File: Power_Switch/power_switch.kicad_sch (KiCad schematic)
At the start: 24 parts, among them J1 Conn_01x03_Pin, J2 GCT_FFC2B28-12-G, J6 Conn_01x02_Pin, Q9 2N7002, SW1 SW_SPDT, U6 BQ24075RGT

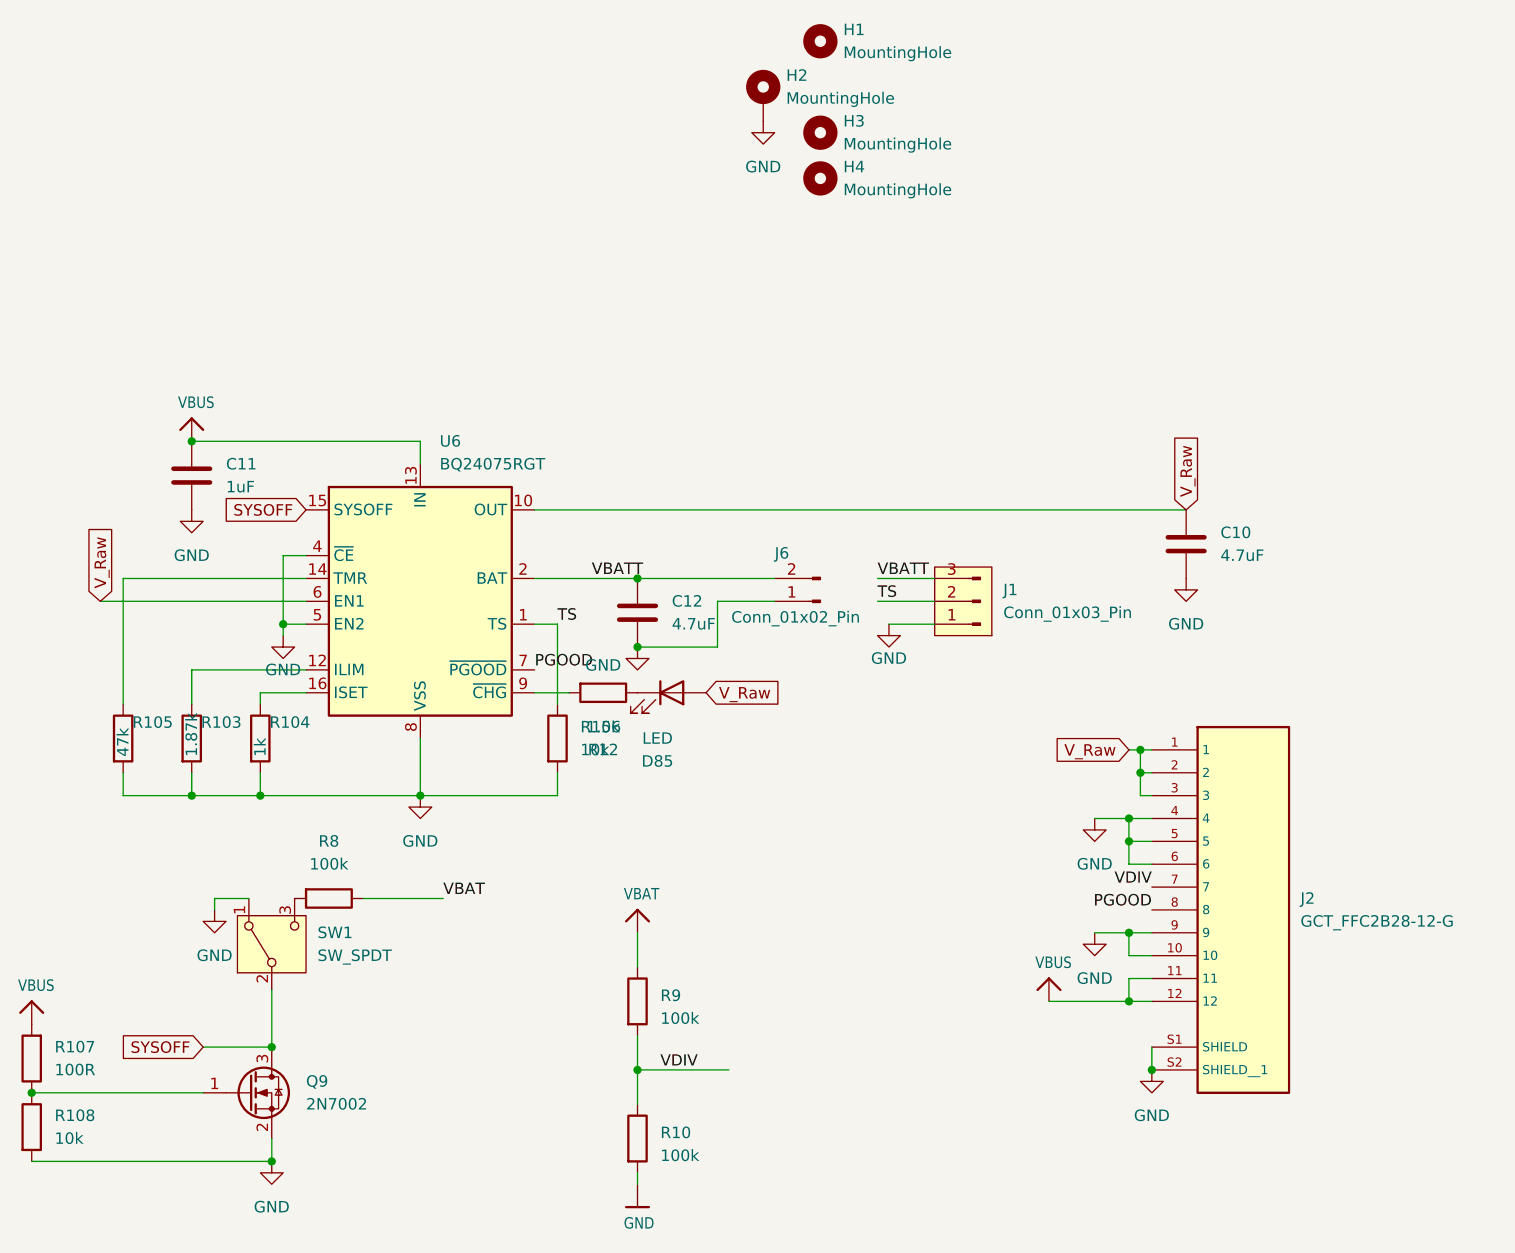
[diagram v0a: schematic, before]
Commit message: Work on Power Switch
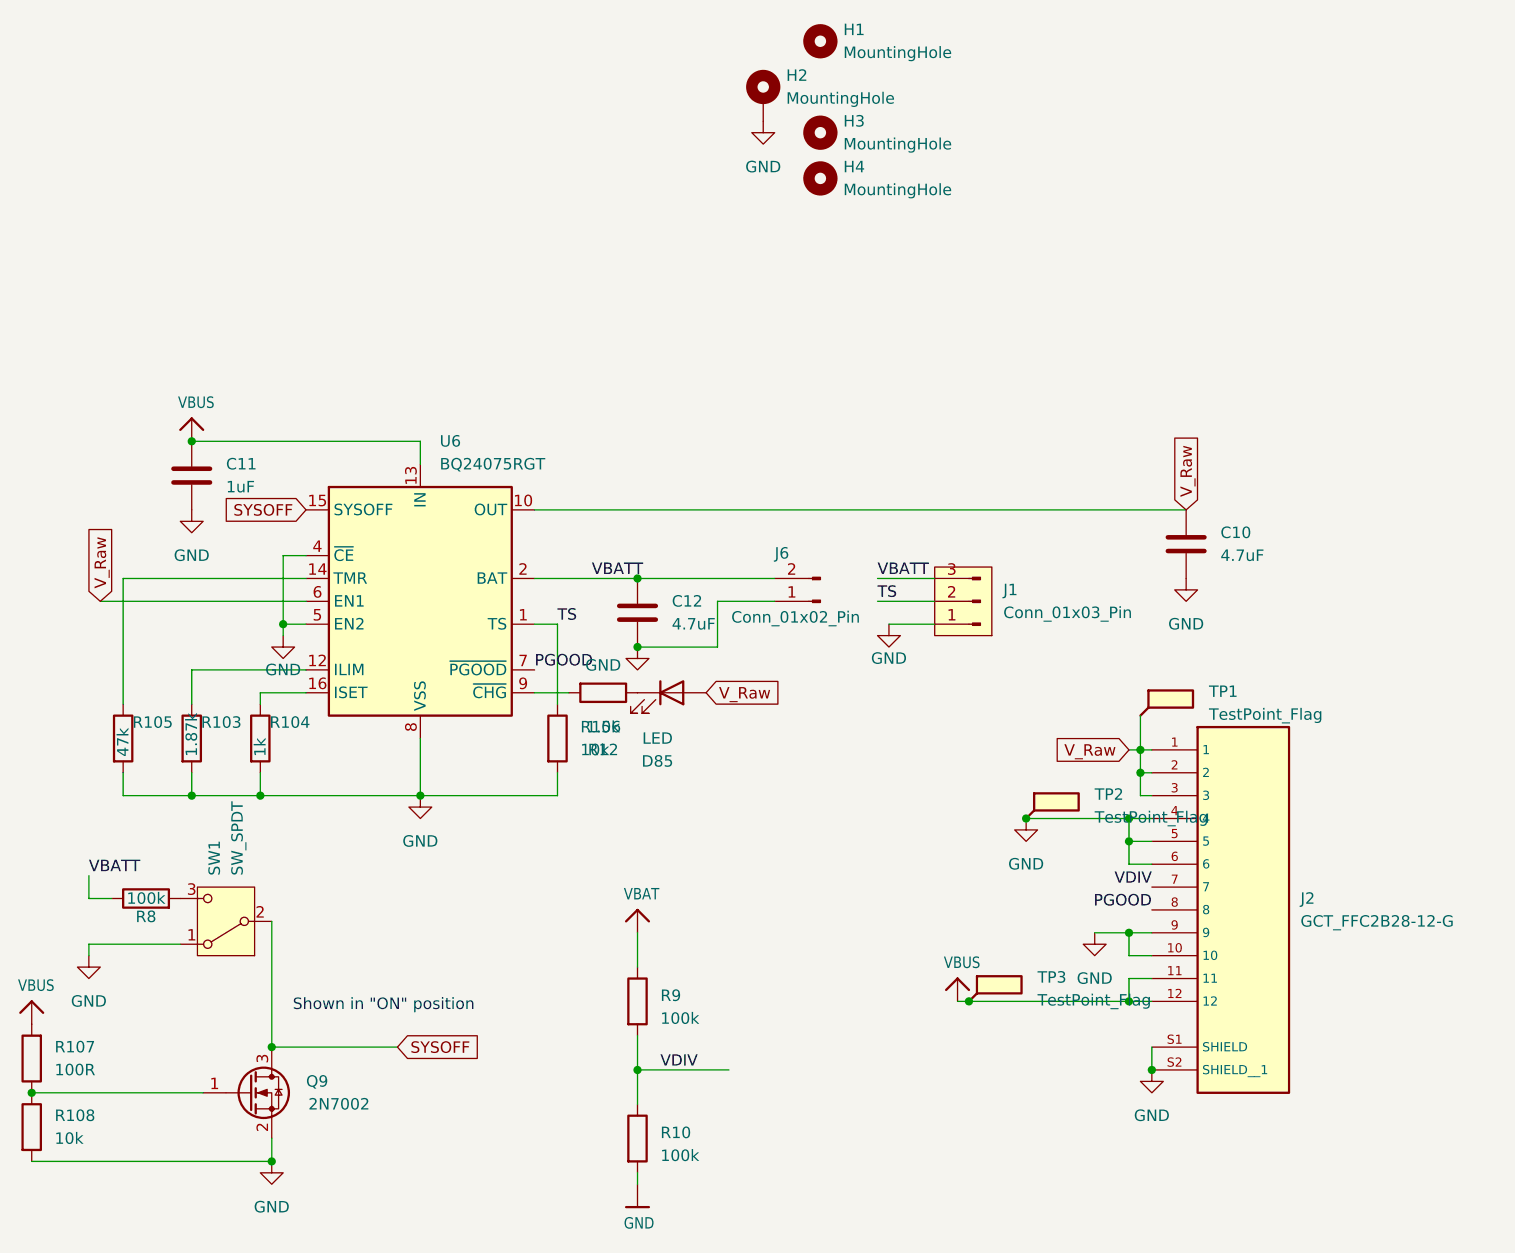
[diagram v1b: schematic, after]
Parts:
- added TP1, TP2, TP3: TestPoint_Flag, TestPoint:TestPoint_Pad_1.5x1.5mm, symbol Connector:TestPoint_Flag
- SW1: footprint JohnDeereLibrary:ET01MD1CBE -> JohnDeereLibrary:ET01M3D1SAPE
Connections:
- net GND: now also TP2.1
- net VBAT: no longer R8.1
- net VBATT: now also R8.1
- net VBUS: now also TP3.1
- net V_Raw: now also TP1.1
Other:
- note added: "Shown in "ON" position"
- moved on the sheet: R8, SW1
